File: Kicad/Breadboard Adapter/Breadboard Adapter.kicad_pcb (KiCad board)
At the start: 2 copper layers, 25.4 x 105.4 mm, 6 parts, among them J1 Bus_ISA_8bit, J2 USB_C_Receptacle_USB2.0, J3 Conn_01x31, J4 Conn_01x31, J9 Bus_ISA_8bit, SW1 SW_Push_DPDT

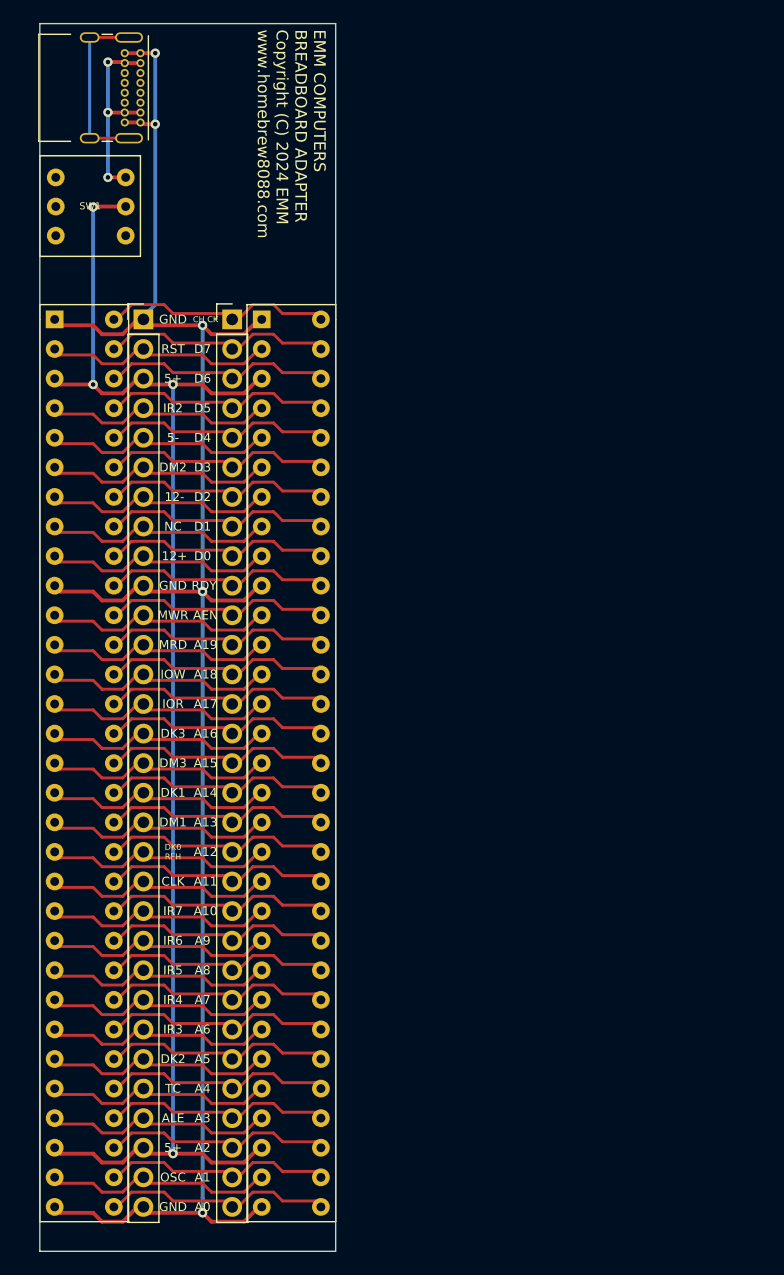
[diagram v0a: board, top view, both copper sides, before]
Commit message: update adapter
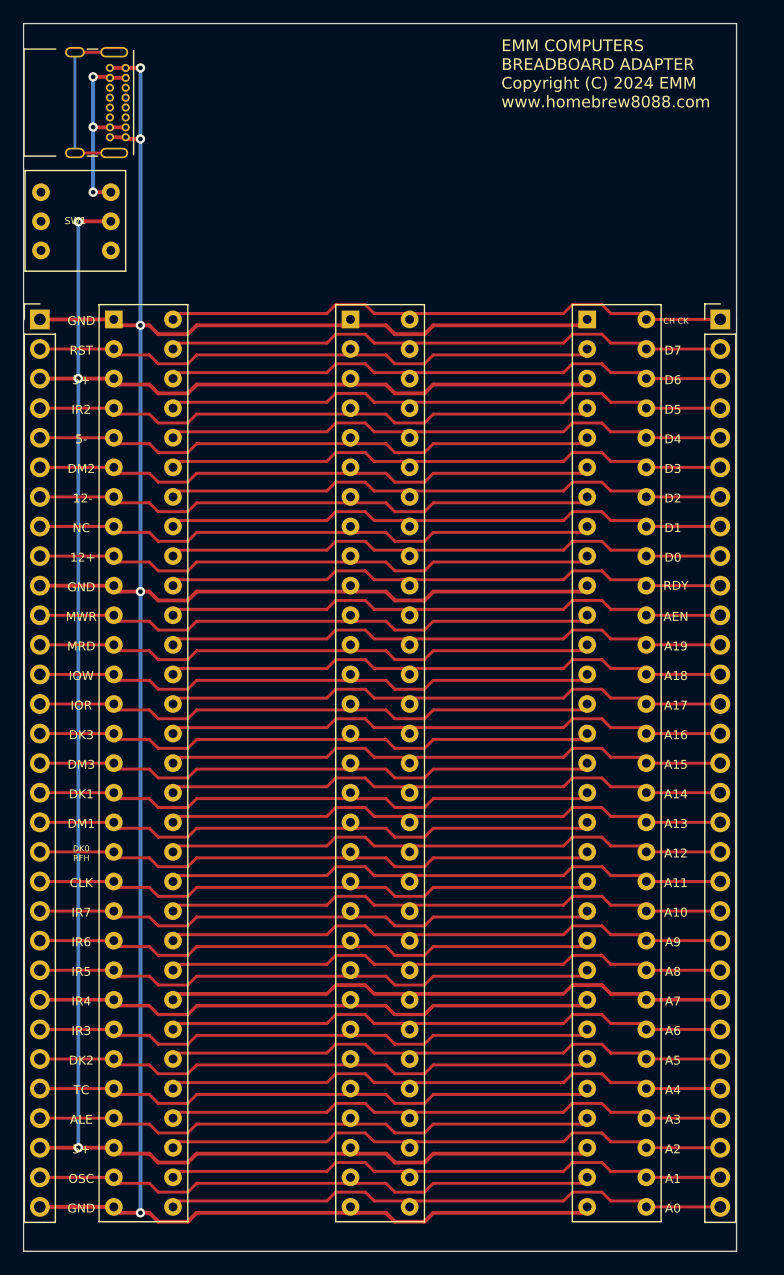
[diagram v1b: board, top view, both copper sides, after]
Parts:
- added J5: Bus_ISA_8bit, My:8-bit-ISA, F.Cu at (116.8, 38.1)
- moved J9 45.7 mm to (137.2, 38.1)
- moved J4 41.9 mm to (148.6, 38.1)
- moved J1 12.7 mm to (96.5, 38.1)
- moved J3 8.89 mm to (90.2, 38.1)
- moved J2 1.80 mm to (97.5, 16.5)
- moved SW1 1.80 mm to (96.3, 32.2)
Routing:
- net /GND: track 164.5 -> 250.9 mm
- net /A7: track 19.9 -> 98.2 mm
- net /IRQ4: track 19.9 -> 98.2 mm
- net /5+: track 123.9 -> 180.5 mm, vias 4 -> 3
- net /A5: track 19.9 -> 49.1 mm
- net /A3: track 19.9 -> 49.1 mm
- net /A10: track 19.9 -> 49.1 mm
- net /D7: track 19.9 -> 49.1 mm
- net /D0: track 19.9 -> 49.1 mm
- net /A9: track 19.9 -> 49.1 mm
- net /A16: track 19.9 -> 49.1 mm
- net /A11: track 19.9 -> 49.1 mm
- net /A0: track 19.9 -> 49.1 mm
- net /A8: track 19.9 -> 49.1 mm
- net /A6: track 19.9 -> 49.1 mm
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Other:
- board size 25.4 x 105.4 mm -> 61.2 x 105.4 mm
